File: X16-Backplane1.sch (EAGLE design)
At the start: 22 parts, among them J1 CONN_PXC-8-RA-1778683, J2 CONN_ET60S-D04-3-08-D04-X-R1-S, J3 SAMTEC-HTST-110-04-X-D-RAJ, J5 SAMTEC-HTST-110-04-X-D-RAJ, U2 TRANS_ULN2003AD

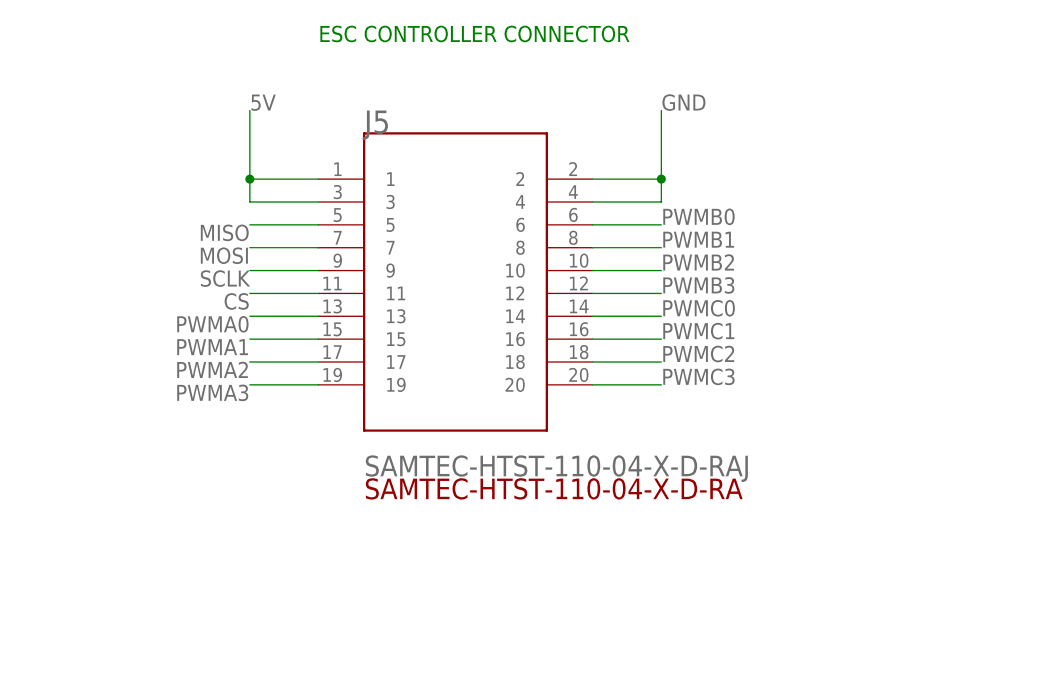
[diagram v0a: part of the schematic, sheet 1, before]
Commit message: Add files via upload
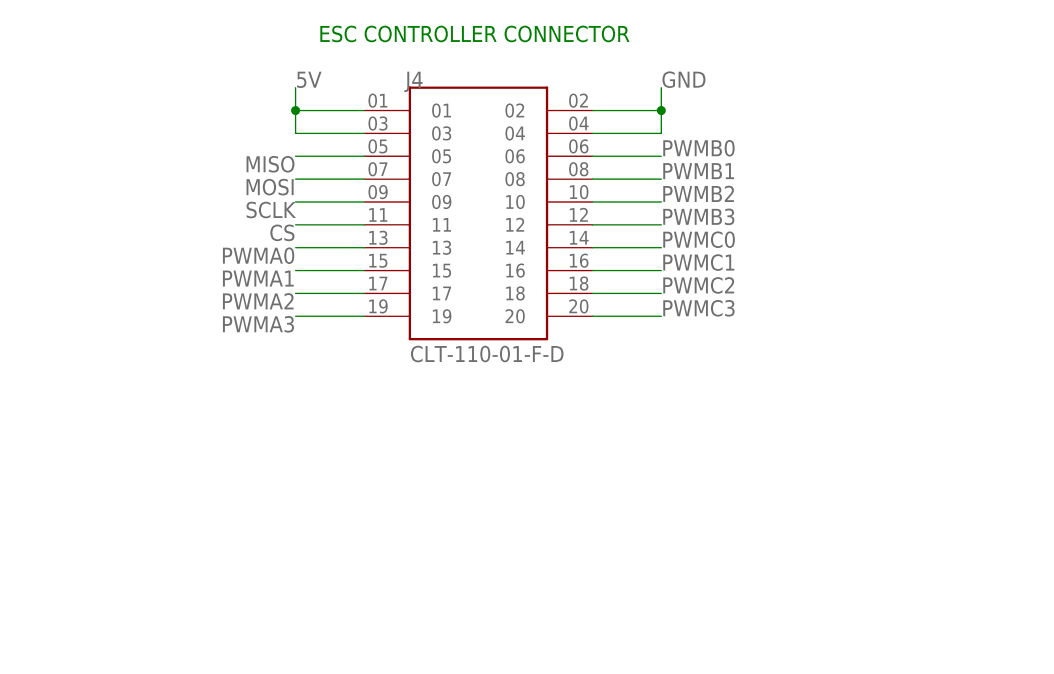
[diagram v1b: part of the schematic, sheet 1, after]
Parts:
- removed J5: SAMTEC-HTST-110-04-X-D-RAJ, X16_Backplane:SAMTEC-HTST-110-04-X-D-RAJ
- added J4: CLT-110-01-F-D, X16_Backplane:CLT-110-01-F-D
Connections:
- net 5V: now also J4.01, J4.03; no longer J5.1, J5.3
- net CS: now also J4.11; no longer J5.11
- net GND: now also J4.02, J4.04; no longer J5.2, J5.4
- net MISO: now also J4.05; no longer J5.5
- net MOSI: now also J4.07; no longer J5.7
- net PWMA0: now also J4.13; no longer J5.13
- net PWMA1: now also J4.15; no longer J5.15
- net PWMA2: now also J4.17; no longer J5.17
- net PWMA3: now also J4.19; no longer J5.19
- net PWMB0: now also J4.06; no longer J5.6
- net PWMB1: now also J4.08; no longer J5.8
- net PWMB2: now also J4.10; no longer J5.10
- net PWMB3: now also J4.12; no longer J5.12
- net PWMC0: now also J4.14; no longer J5.14
- net PWMC1: now also J4.16; no longer J5.16
- net PWMC2: now also J4.18; no longer J5.18
- net PWMC3: now also J4.20; no longer J5.20
- net SCLK: now also J4.09; no longer J5.9
